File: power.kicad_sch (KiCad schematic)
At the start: 47 parts, among them J10 Conn_01x02_Pin, Q2 DMG2301L, U12 TPS63061, U13 LTC4412xS6, U14 TPS61092, U15 AP2112K-3.3, U16 TPS61092, U9 TPS82130

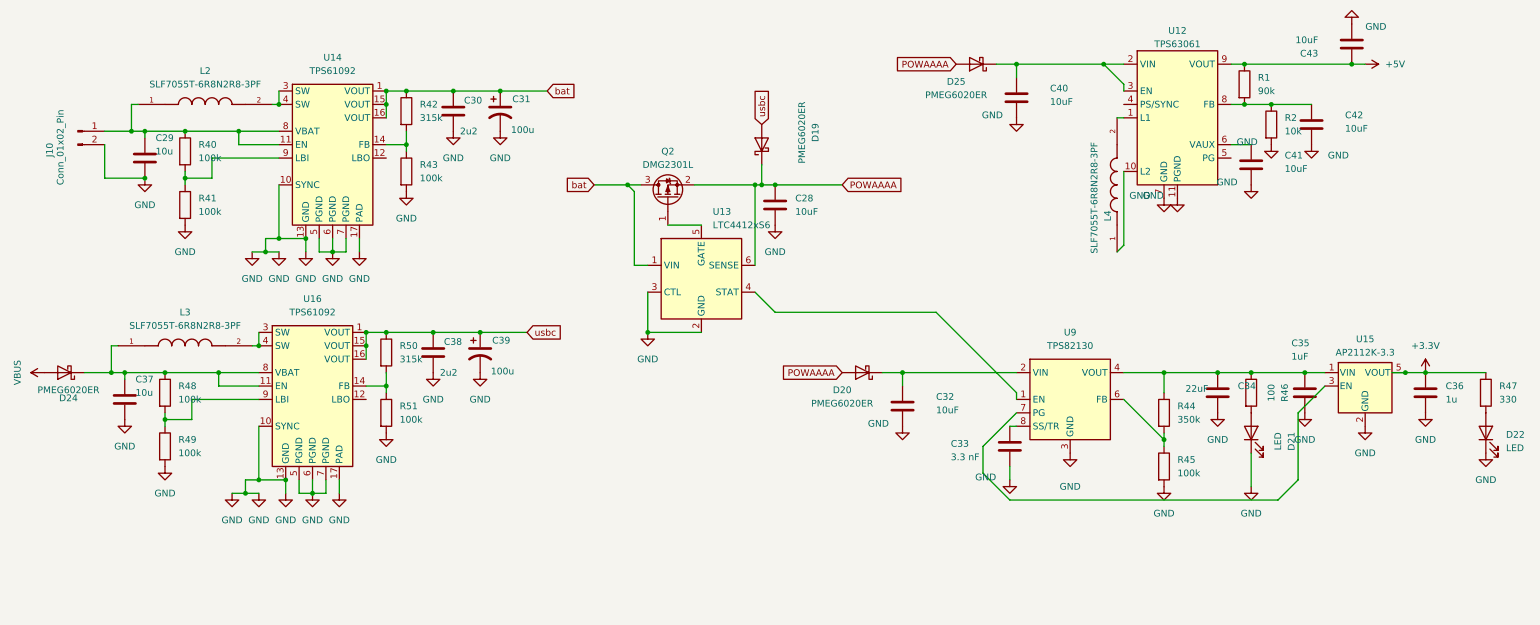
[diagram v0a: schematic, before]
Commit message: Changes, idr what though :(
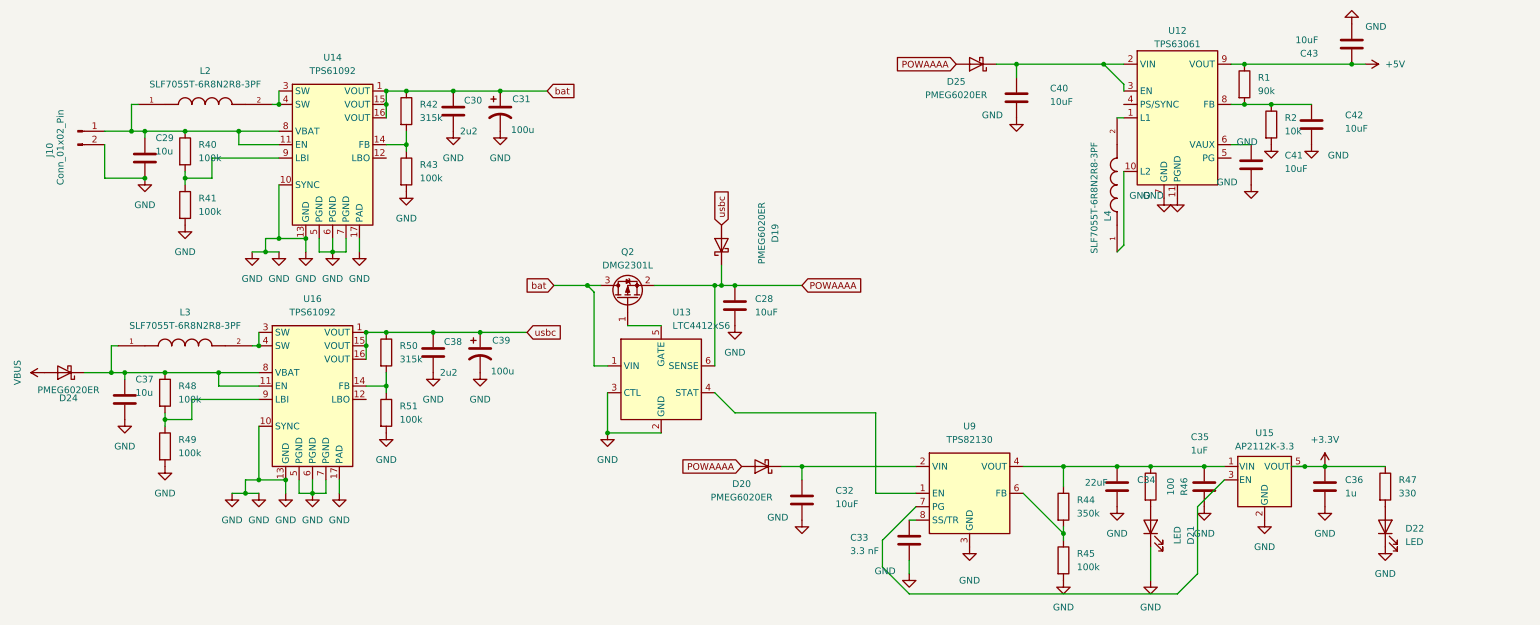
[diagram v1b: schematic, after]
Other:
- moved on the sheet: C28, C32, C33, C34, C35, C36, D19, D20, D21, D22, Q2, R44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
